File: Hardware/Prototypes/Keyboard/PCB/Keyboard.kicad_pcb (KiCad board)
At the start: 2 copper layers, 44.2 x 18.5 mm, 20 parts, among them U1 ATMEGA32U4-QFN44, X1 ABM10-16.000MHZ-D30-T3

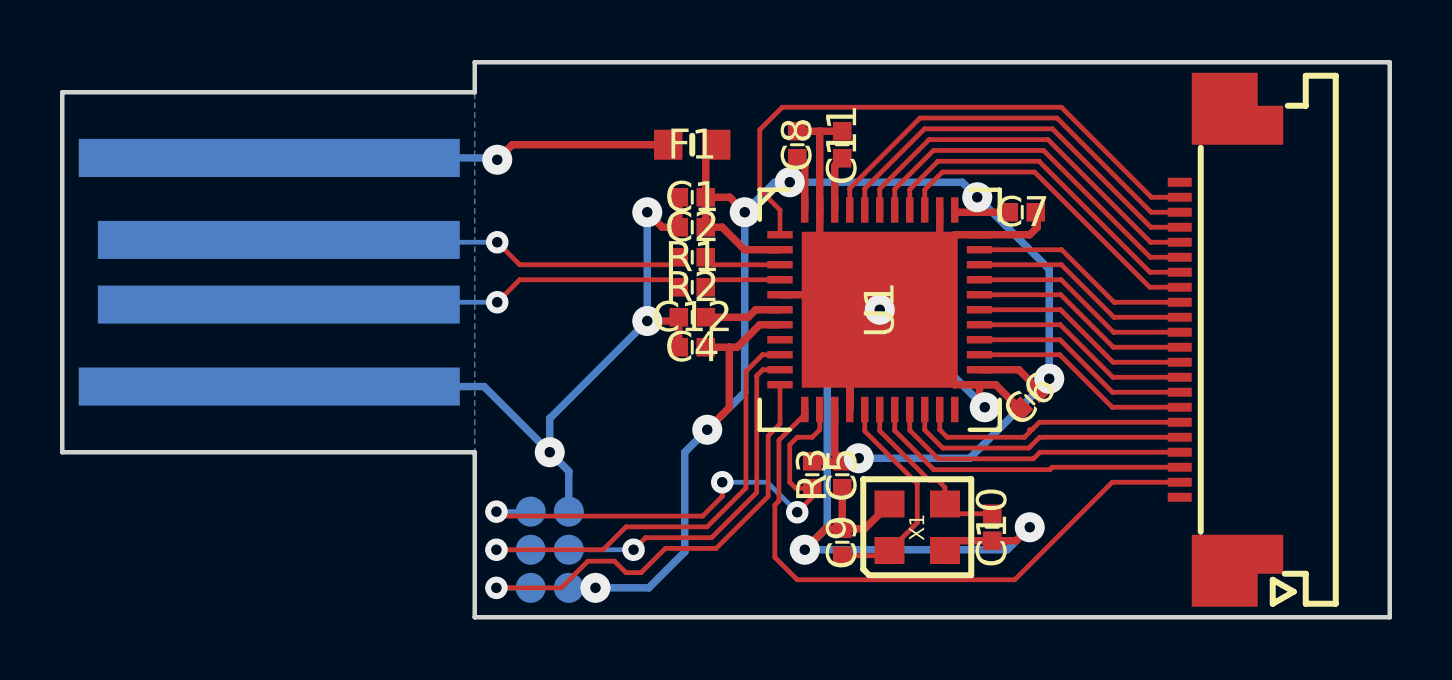
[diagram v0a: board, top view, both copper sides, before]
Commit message: Keyboard update
Version 1.1
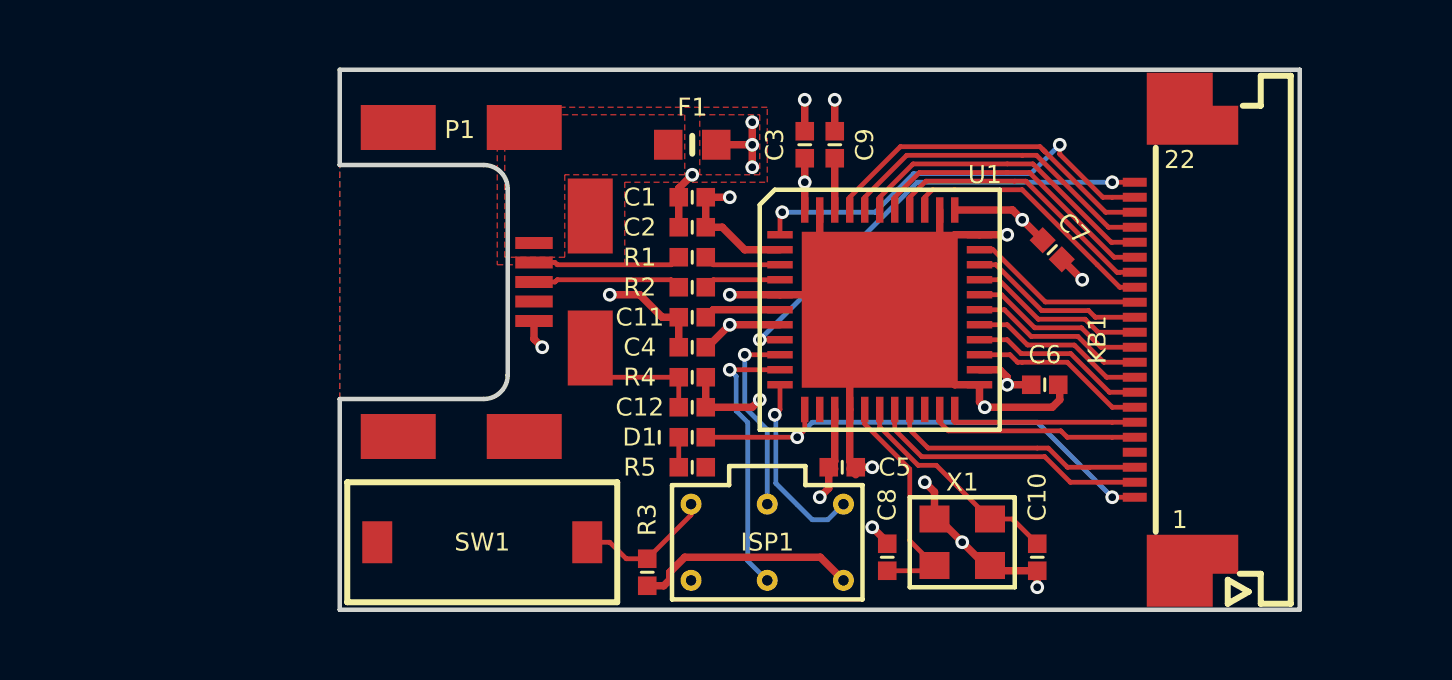
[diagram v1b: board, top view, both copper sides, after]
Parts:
- removed USB1: TO HOST, Edge-Connectors:USB_EDGE
- added C3: 100n, SMD-DiscreteB:C-0402-1005, F.Cu at (160.5, 100.5)
- added D1: STATUS, SMD-DiscreteB:LED-0402-1005, F.Cu at (156.8, 110.2)
- added P1: USB_OTG, SMD-Connectors:USB-MICRO-MOLEX-47491-0001, F.Cu at (145.0, 105.1)
- added R4: 1M, SMD-DiscreteB:R-0402-1005, F.Cu at (156.8, 108.2)
- added R5: 1k, SMD-DiscreteB:R-0402-1005, F.Cu at (156.8, 111.2)
- added SW1: RESET, SMD-Switches:KSR251GLFS, F.Cu at (149.8, 113.8)
- C10: value 10p -> 15p
- C11: value 100n -> 1µ
- C12: value 1µ -> 4n7
- C8: value 100n -> 15p
- C9: value 10p -> 100n
- F1: footprint SMD-DiscreteB:0603-1608 -> SMD-DiscreteB:F-0603-1608
- ISP1: footprint SMD-Connectors:ISP-PADS_1mm27 -> SMD-Connectors:ISP-PADS_2mm54; moved to F.Cu
- moved C8 14.1 mm to (163.2, 114.2)
- moved C9 13.3 mm to (161.5, 100.5)
- moved C11 7.62 mm to (156.8, 106.2), turned to 180 degrees
- moved ISP1 7.25 mm to (159.2, 113.8), turned to 180 degrees
- moved R3 6.39 mm to (155.2, 114.8), turned to 90 degrees
- moved C12 3.00 mm to (156.8, 109.2)
- moved C10 1.80 mm to (168.2, 114.2)
- moved C7 1.60 mm to (168.8, 104.0), turned to 315 degrees
- moved X1 1.58 mm to (165.8, 113.8)
- moved KB1 1.50 mm to (171.5, 107.0)
- moved C6 0.71 mm to (168.5, 108.5), turned to 0 degrees
- moved C5 0.25 mm to (161.8, 111.2), turned to 0 degrees
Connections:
- C11 pad 1: /VARef -> /VUCap
- C12 pad 1: /VUCap -> GND
- C12 pad 2: GND -> GNDPWR
- C8 pad 1: +5V -> Net-(C8-Pad1)
- C9 pad 1: Net-(C9-Pad1) -> /VARef
- KB1 pad 1: (no net) -> /LED
- KB1 pad 22: (no net) -> /TMP
- KB1 pad 4: /COL_11 -> /COL_10
- KB1 pad 5: /COL_10 -> /COL_11
- U1 pad 12: /COL_9 -> /LED
- U1 pad 16: Net-(C9-Pad1) -> Net-(C8-Pad1)
- U1 pad 18: /COL_12 -> /COL_9
- U1 pad 19: /COL_11 -> /COL_12
- U1 pad 21: /COL_8 -> /COL_11
- U1 pad 22: (no net) -> /COL_8
- U1 pad 8: (no net) -> /TMP
- X1 pad 1: Net-(C9-Pad1) -> Net-(C8-Pad1)
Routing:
- net GND: track 117.9 -> 53.3 mm, vias 7 -> 15
- net +5V: track 63.4 -> 28.0 mm, vias 7 -> 9
- net /LED: track 0.00 -> 16.6 mm, vias 0 -> 2
- net /TMP: track 0.00 -> 15.3 mm, vias 0 -> 2
- net +5VD: track 13.0 -> 0.00 mm, vias 1 -> 0
- net /RESET: track 17.4 -> 4.65 mm, vias 3 -> 0
- net /COL_9: track 20.8 -> 9.79 mm
- net /COL_10: track 9.58 -> 0.00 mm
- net /MISO: track 15.7 -> 6.35 mm
- net /SCK: track 15.6 -> 6.52 mm
- net Net-(P1-Pad2): track 13.7 -> 5.21 mm, vias 1 -> 0
- net Net-(P1-Pad3): track 13.5 -> 5.21 mm, vias 1 -> 0
- net Net-(C8-Pad1): track 0.00 -> 7.81 mm
- net Net-(C9-Pad1): track 7.46 -> 0.00 mm
- net GNDPWR: track 0.00 -> 5.58 mm
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- added copper zone on F.Cu, net +5V
- added copper zone on Supply.Cu, net +5V
- added copper zone on F.Cu, net +5VD
- added copper zone on F.Cu, net GND
- added copper zone on Ground.Cu, net GND
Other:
- board size 44.2 x 18.5 mm -> 32 x 18 mm
- copper layers 2 -> 4
- net class Default: clearance 0.2 -> 0.127; via_dia 0.75 -> 0.4572; via_drill 0.35 -> 0.254
- net class Power: clearance 0.2 -> 0.127; via_dia 1 -> 0.4572; via_drill 0.5 -> 0.254
- rule trace_clearance: 0.2 -> 0.127
- rule trace_min: 0.1524 -> 0.127
- rule via_min_drill: 0.3302 -> 0.254
- rule via_min_size: 0.6858 -> 0.4572
- board text added: "1"
- board text added: "22"
- board text added: "USB Keyboard v1.1 RasmusB 2016 Psion Series 5/5mx"
- board text removed: "USB Keyboard RasmusB 2015 for Psion Series 5/5mx"
- board text removed: "v1.0"
